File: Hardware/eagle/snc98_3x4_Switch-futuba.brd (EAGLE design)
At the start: 56.4 x 83.2 mm, 73 parts

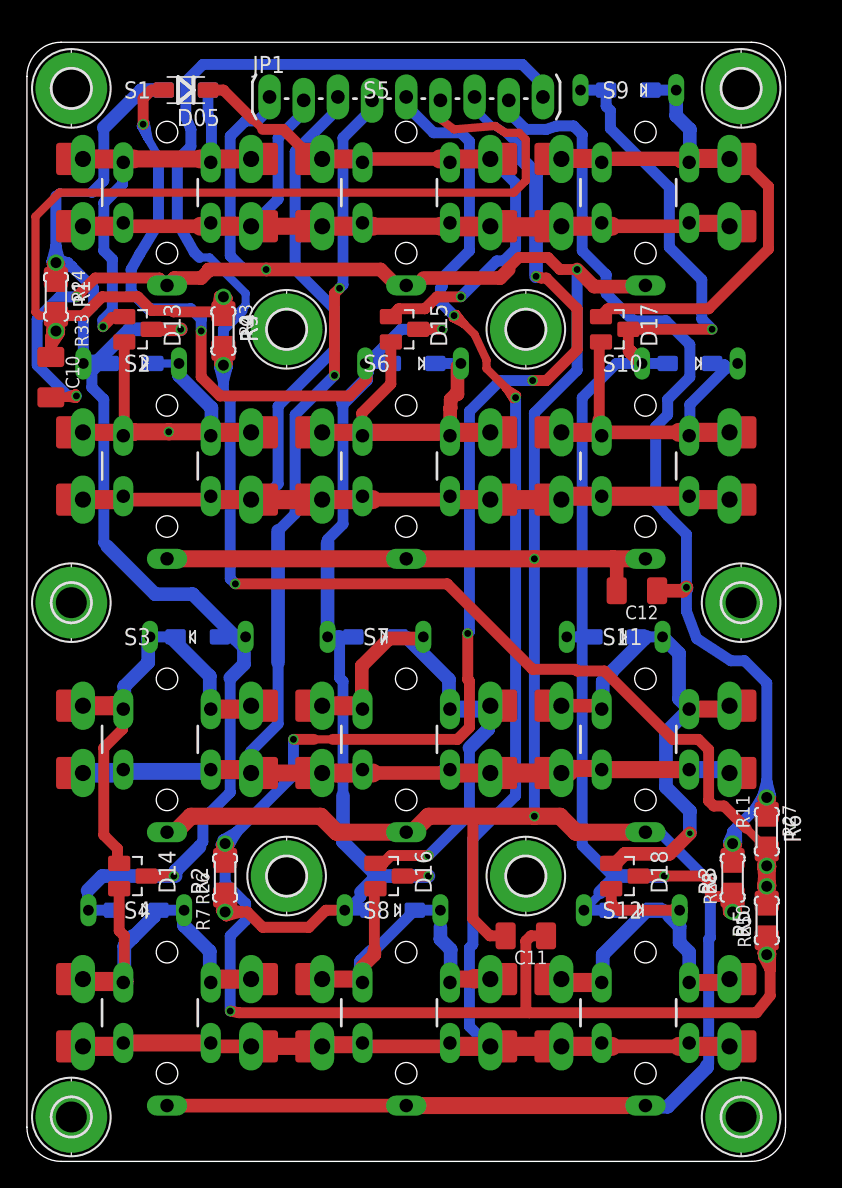
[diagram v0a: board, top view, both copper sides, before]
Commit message: add_prozent
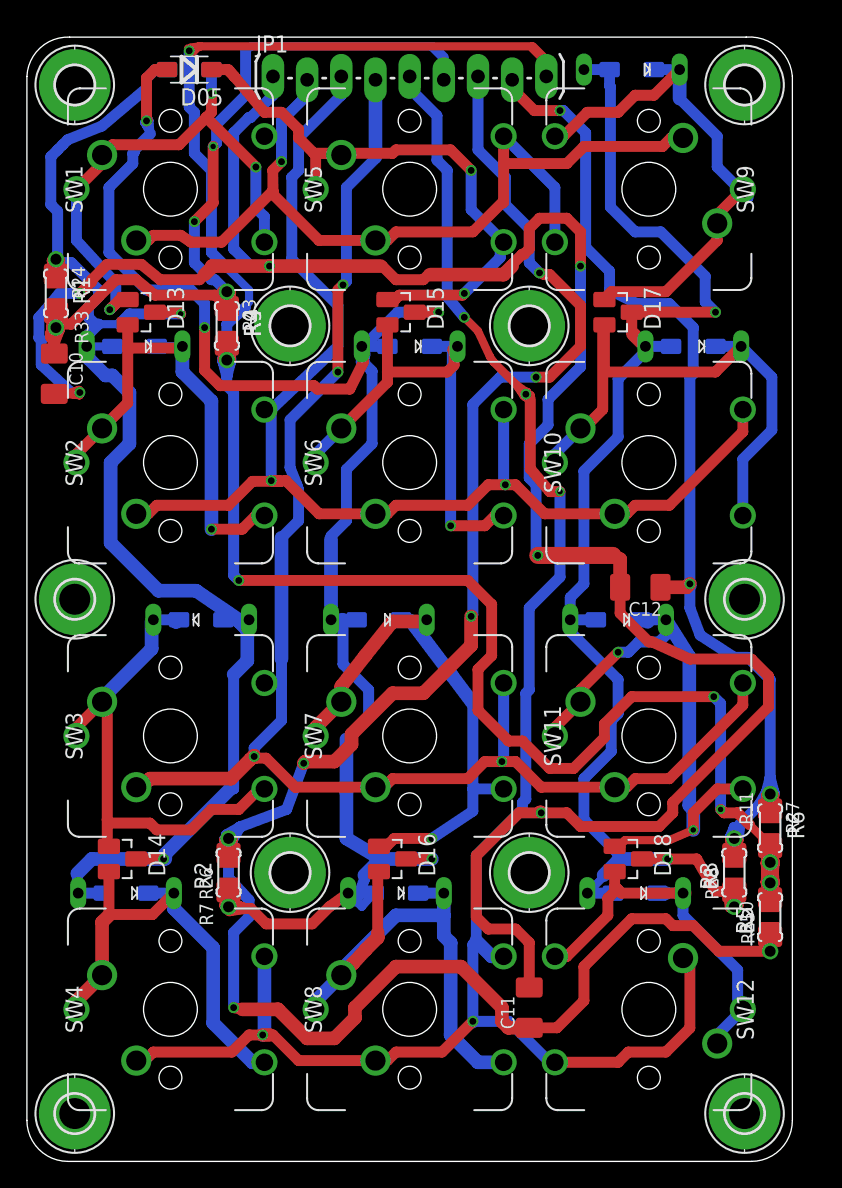
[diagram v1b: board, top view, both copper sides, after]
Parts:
- removed S1, S10, S11, S12, S2, S3, S4, S5, S6, S7, S8, S9: B3F-4150, SmartPrj:TACTILE-PTH-12MM
- added SW1, SW10, SW11, SW12, SW2, SW3, SW4, SW5, SW6, SW7, SW8, SW9: CHERRY_MX_WITH_FIXING_PINS, Cherry_MX_v7.0:MX1A-XXNW
- moved C11 5.34 mm to (37.3, 11.4), turned to 90 degrees
- moved JP1 1.55 mm to (18.3, 80.5)
- moved D01 1.55 mm to (12.1, 81.2)
- moved D05 1.55 mm to (12.1, 81.2)
- moved D09 1.55 mm to (45.0, 81.2)
- moved D25 1.55 mm to (45.0, 81.2)
- moved D04 1.48 mm to (7.37, 19.9)
- moved D21 1.48 mm to (7.37, 19.9)
- moved D14 1.48 mm to (7.11, 22.5)
- moved D03 1.30 mm to (13.0, 40.3)
- moved D06 1.30 mm to (28.4, 60.6)
- moved D15 1.30 mm to (27.8, 63.1)
- moved D20 1.30 mm to (13.0, 40.3)
- moved D22 1.30 mm to (28.4, 60.6)
- moved D02 1.30 mm to (8.00, 60.6)
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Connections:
- net C1: now also SW1.1, SW1.3, SW5.1, SW5.3, SW9.1, SW9.3; no longer S1.P$1, S1.P$11, S1.P$12, S1.P$2, S1.P$21, S1.P$22, S5.P$1, S5.P$11, S5.P$12, S5.P$2, S5.P$21, S5.P$22, S9.P$1, S9.P$11, S9.P$12, S9.P$2, S9.P$21, S9.P$22
- net C2: now also SW10.1, SW10.3, SW2.1, SW2.3, SW6.1, SW6.3; no longer S10.P$1, S10.P$11, S10.P$12, S10.P$2, S10.P$21, S10.P$22, S2.P$1, S2.P$11, S2.P$12, S2.P$2, S2.P$21, S2.P$22, S6.P$1, S6.P$11, S6.P$12, S6.P$2, S6.P$21, S6.P$22
- net C3: now also SW11.1, SW11.3, SW3.1, SW3.3, SW7.1, SW7.3; no longer S11.P$1, S11.P$11, S11.P$12, S11.P$2, S11.P$21, S11.P$22, S3.P$1, S3.P$11, S3.P$12, S3.P$2, S3.P$21, S3.P$22, S7.P$1, S7.P$11, S7.P$12, S7.P$2, S7.P$21, S7.P$22
- net C4: now also SW12.1, SW12.3, SW4.1, SW4.3, SW8.1, SW8.3; no longer S12.P$1, S12.P$11, S12.P$12, S12.P$2, S12.P$21, S12.P$22, S4.P$1, S4.P$11, S4.P$12, S4.P$2, S4.P$21, S4.P$22, S8.P$1, S8.P$11, S8.P$12, S8.P$2, S8.P$21, S8.P$22
- net GND: no longer S1.P$15, S10.P$15, S11.P$15, S12.P$15, S2.P$15, S3.P$15, S4.P$15, S5.P$15, S6.P$15, S7.P$15, S8.P$15, S9.P$15
- net N$16: now also SW9.2, SW9.4, SW9.5; no longer S9.P$13, S9.P$14, S9.P$23, S9.P$24, S9.P$3, S9.P$4
- net N$18: now also SW10.2, SW10.4, SW10.5; no longer S10.P$13, S10.P$14, S10.P$23, S10.P$24, S10.P$3, S10.P$4
- net N$19: now also SW2.2, SW2.4, SW2.5; no longer S2.P$13, S2.P$14, S2.P$23, S2.P$24, S2.P$3, S2.P$4
- net N$2: now also SW4.2, SW4.4, SW4.5; no longer S4.P$13, S4.P$14, S4.P$23, S4.P$24, S4.P$3, S4.P$4
- net N$21: now also SW11.2, SW11.4, SW11.5; no longer S11.P$13, S11.P$14, S11.P$23, S11.P$24, S11.P$3, S11.P$4
- net N$22: now also SW12.2, SW12.4, SW12.5; no longer S12.P$13, S12.P$14, S12.P$23, S12.P$24, S12.P$3, S12.P$4
- net N$24: now also SW5.2, SW5.4, SW5.5; no longer S5.P$13, S5.P$14, S5.P$23, S5.P$24, S5.P$3, S5.P$4
- net N$25: now also SW6.2, SW6.4, SW6.5; no longer S6.P$13, S6.P$14, S6.P$23, S6.P$24, S6.P$3, S6.P$4
- net N$28: now also SW7.2, SW7.4, SW7.5; no longer S7.P$13, S7.P$14, S7.P$23, S7.P$24, S7.P$3, S7.P$4
- net N$30: now also SW8.2, SW8.4, SW8.5; no longer S8.P$13, S8.P$14, S8.P$23, S8.P$24, S8.P$3, S8.P$4
- net N$32: now also SW3.2, SW3.4, SW3.5; no longer S3.P$13, S3.P$14, S3.P$23, S3.P$24, S3.P$3, S3.P$4
- net N$6: now also SW1.2, SW1.4, SW1.5; no longer S1.P$13, S1.P$14, S1.P$23, S1.P$24, S1.P$3, S1.P$4
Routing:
- net GND: track 272.0 -> 169.2 mm
- net C4: track 162.6 -> 142.2 mm, vias 2 -> 5
- net A1: track 94.4 -> 76.0 mm, vias 0 -> 2
- net AREF: track 173.0 -> 187.8 mm, vias 1 -> 4
- net N$16: track 54.9 -> 40.5 mm
- net N$18: track 31.1 -> 42.5 mm
- net A_1: track 120.9 -> 110.0 mm
- net A2: track 168.0 -> 158.3 mm
- net N$30: track 32.0 -> 40.9 mm
- net C3: track 123.7 -> 114.9 mm, vias 2 -> 4
- net C2: track 89.1 -> 95.8 mm, vias 0 -> 2
- net N$19: track 31.1 -> 36.7 mm
- net A_2: track 132.3 -> 137.7 mm
- net N$25: track 35.1 -> 38.8 mm, vias 0 -> 1
- net N$28: track 45.7 -> 42.2 mm
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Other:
- board size 56.4 x 83.2 mm -> 56.9 x 83.6 mm
